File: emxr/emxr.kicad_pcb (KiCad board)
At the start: 2 copper layers, 170.2 x 76.5 mm, 137 parts, among them IC201 NJM4558D, IC301 NJM4556D, IC401 NJM2068DD, IC402 NJM4580, IC501 NJM2068DD, IC502 NJM4580, J101 POWER, J103 Bus Conn, J104 GEQ_L_PRE, J105 GEQ_L_POST, J106 GEQ_R_PRE, J107 GEQ_R_POST, J108 AUDIO_OUT, J205 InpVolL, J206 InpVolR, J208 SrcSel, J301 HPHONES, J302 HPVolL, J303 HPVolR, J401 FrontVolL, J501 FrontVolL

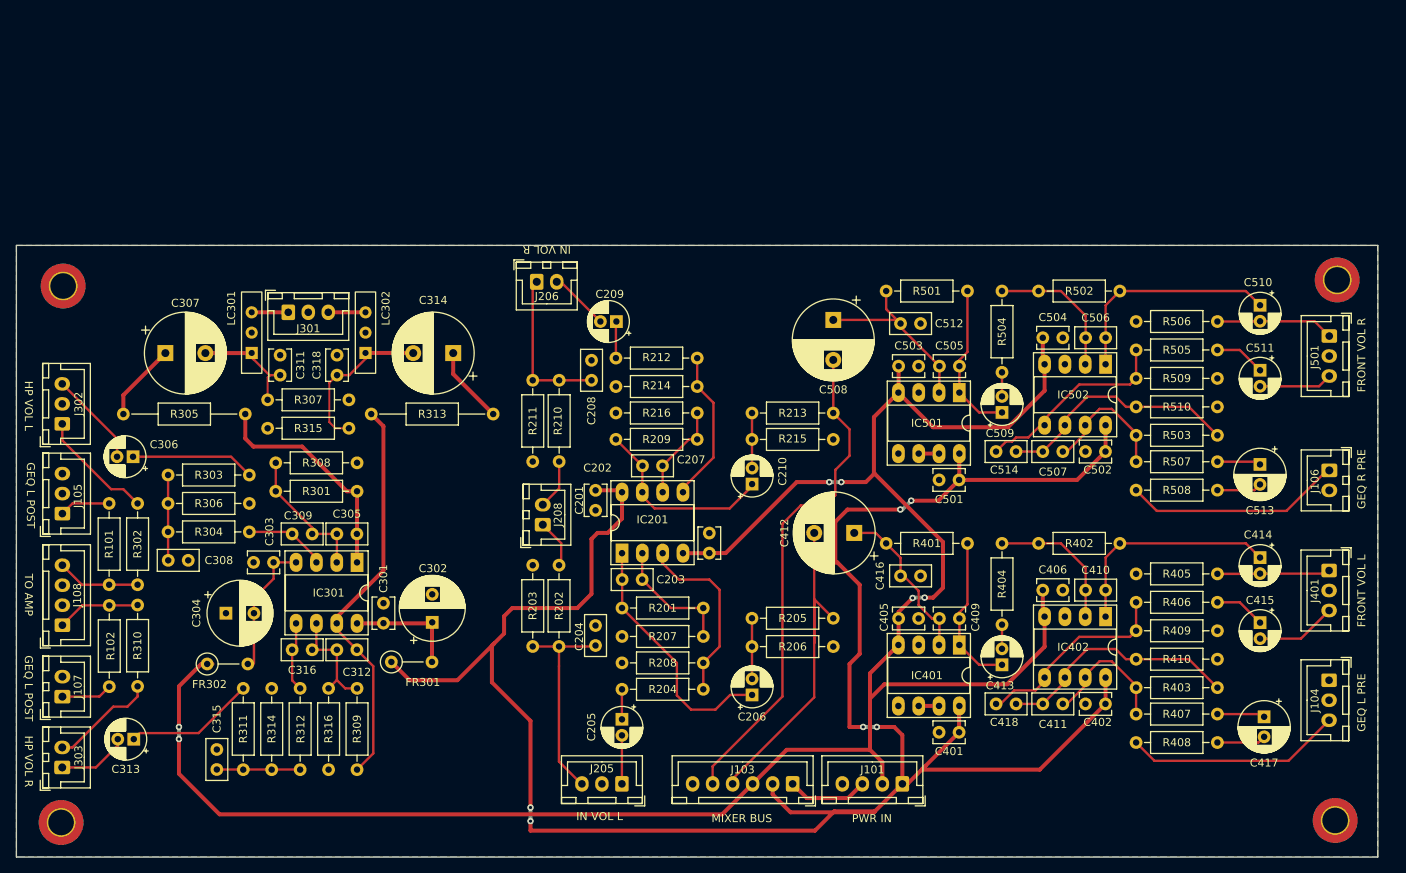
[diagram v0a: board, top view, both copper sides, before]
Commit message: more cleaning up/finishing touches
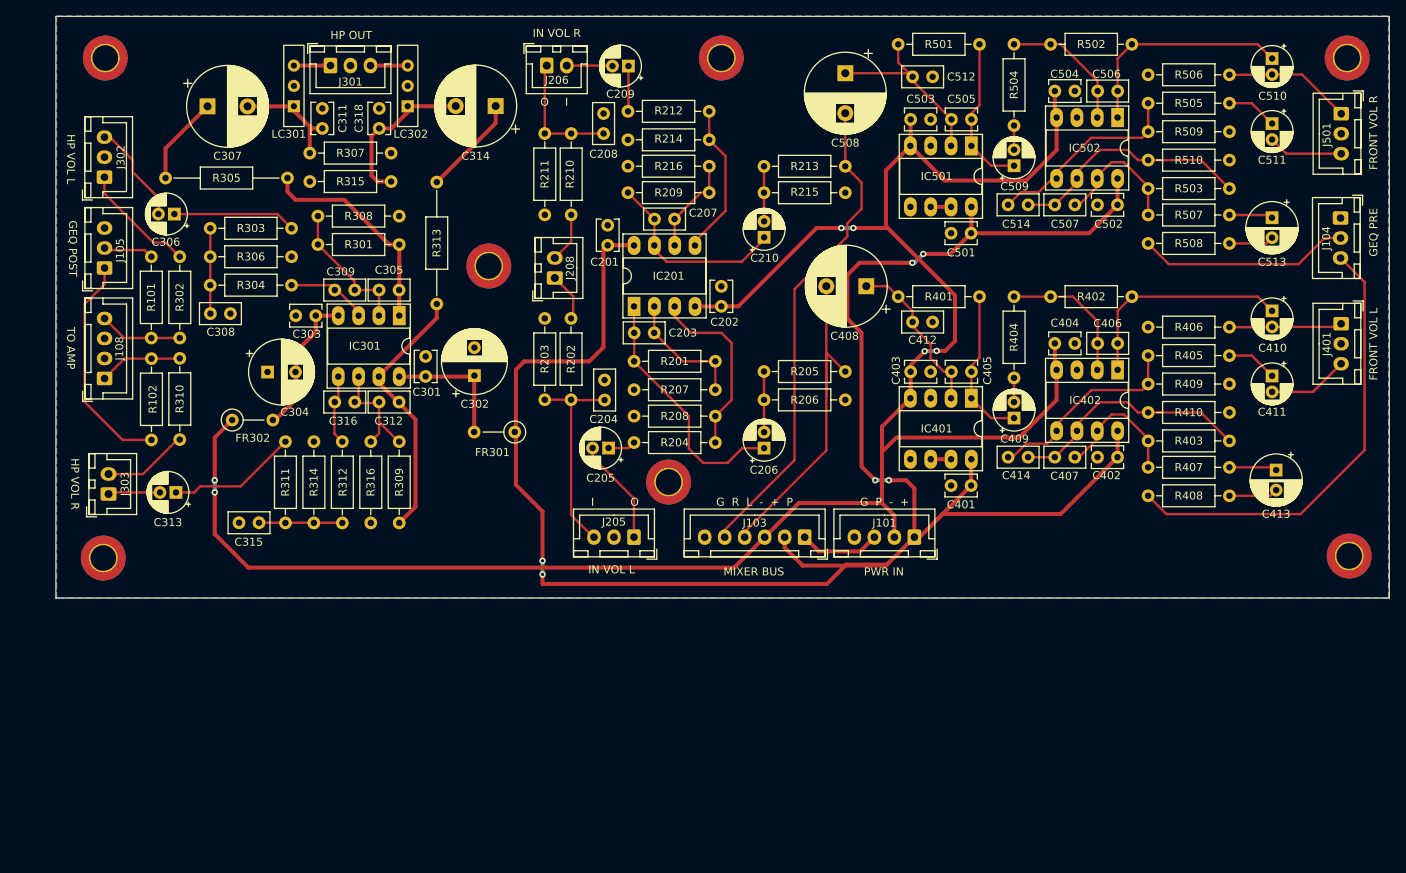
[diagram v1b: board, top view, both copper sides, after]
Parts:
- removed J106: GEQ_R_PRE, Connector_JST:JST_XH_B2B-XH-A_1x02_P2.50mm_Vertical
- removed J107: GEQ_R_POST, Connector_JST:JST_XH_B2B-XH-A_1x02_P2.50mm_Vertical
- added H105: MH, MountingHole:MountingHole_3.2mm_M3_DIN965_Pad_TopBottom, F.Cu at (150.1, 66.8)
- added H106: MH, MountingHole:MountingHole_3.2mm_M3_DIN965_Pad_TopBottom, F.Cu at (143.5, 119.8)
- added H107: MH, MountingHole:MountingHole_3.2mm_M3_DIN965_Pad_TopBottom, F.Cu at (121.0, 92.8)
- J104: value GEQ_L_PRE -> GEQ_PRE
- J105: value GEQ_L_POST -> GEQ_POST
- moved J104 57.8 mm to (227.5, 86.8)
- moved C201 35.7 mm to (135.9, 87.7), turned to -90 degrees
- moved J303 34.7 mm to (73.5, 121.2)
- moved C205 34.0 mm to (136.0, 115.5), turned to 180 degrees
- moved H104 33.5 mm to (72.8, 129.2)
- moved H103 33.1 mm to (228.6, 129.0)
- moved FR301 32.6 mm to (124.3, 113.5), turned to 180 degrees
- moved C209 32.0 mm to (138.5, 67.8)
- moved C412 31.8 mm to (174.0, 99.8)
- moved C316 31.4 mm to (101.8, 109.8)
- moved C312 31.4 mm to (107.3, 109.8)
- moved C314 31.3 mm to (121.9, 72.8)
- moved C301 31.3 mm to (113.1, 104.1)
- moved LC301 31.3 mm to (96.7, 70.2)
- moved C303 31.3 mm to (99.4, 99.0)
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- renumbered C405 to C403, C406 to C404, C409 to C405, C410 to C406, C411 to C407, C412 to C408, C413 to C409, C414 to C410, C415 to C411, C416 to C412, C417 to C413, C418 to C414, R406 to R405, R405 to R406
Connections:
- J104 pad 2: unconnected-(J104-Pad2) -> SINGAL_R_PRE_GEQ
- J105 pad 2: unconnected-(J105-Pad2) -> Net-(J105-Pad2)
- R101 pad 1: Net-(J105-Pad1) -> Net-(J105-Pad2)
- R102 pad 1: Net-(J107-Pad1) -> Net-(J105-Pad1)
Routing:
- net SINGAL_L_PRE_GEQ: track 27.2 -> 56.6 mm
- net +15V: track 267.7 -> 245.1 mm
- net Net-(J105-Pad1): track 6.37 -> 28.2 mm
- net Net-(C312-Pad2): track 50.2 -> 33.1 mm
- net Net-(C205-Pad2): track 6.07 -> 13.3 mm
- net Net-(J107-Pad1): track 6.38 -> 0.00 mm
- net Net-(J105-Pad2): track 0.00 -> 6.35 mm
- net -15V: track 259.5 -> 255.5 mm
- net Net-(C208-Pad1): track 19.9 -> 15.9 mm
- net Net-(C314-Pad1): track 9.69 -> 12.6 mm
- net Net-(J303-Pad2): track 13.3 -> 10.7 mm
- net Net-(C313-Pad2): track 8.87 -> 6.51 mm
- net BUS_R: track 62.7 -> 60.9 mm
- net Net-(C209-Pad2): track 7.51 -> 5.73 mm
- net Net-(C303-Pad1): track 16.6 -> 18.3 mm
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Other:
- board size 170.2 x 76.5 mm -> 166.7 x 72.7 mm
- rule pad_to_mask_clearance: 0 -> 0.2
- board text added: "G P - +"
- board text added: "G R L - + P"
- board text added: "GEQ POST"
- board text added: "GEQ PRE"
- board text added: "HP OUT"
- board text added: "I"
- board text added: "O"
- board text removed: "GEQ L POST"
- board text removed: "GEQ L PRE"
- board text removed: "GEQ R PRE"
